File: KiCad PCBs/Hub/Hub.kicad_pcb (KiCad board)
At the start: 2 copper layers, 113.7 x 55.2 mm, 31 parts, among them J1 Conn_02x04_Top_Bottom, J2 Conn_02x04_Top_Bottom, U1 L7805CV

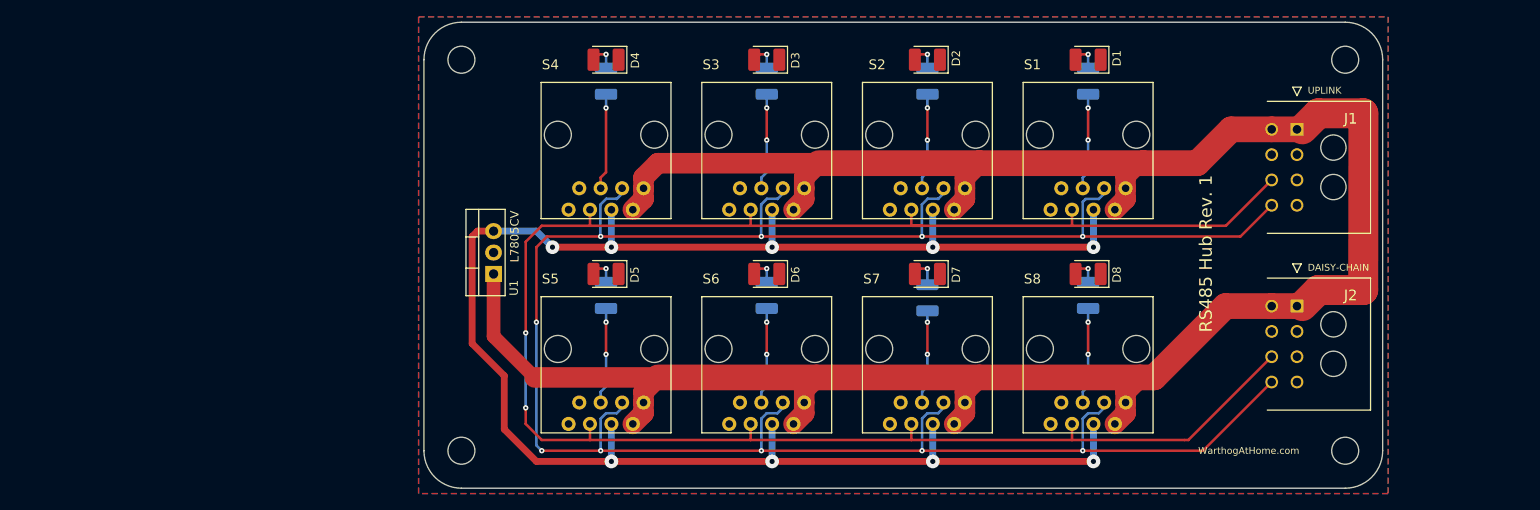
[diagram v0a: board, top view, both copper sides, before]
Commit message: First version of Hub completed
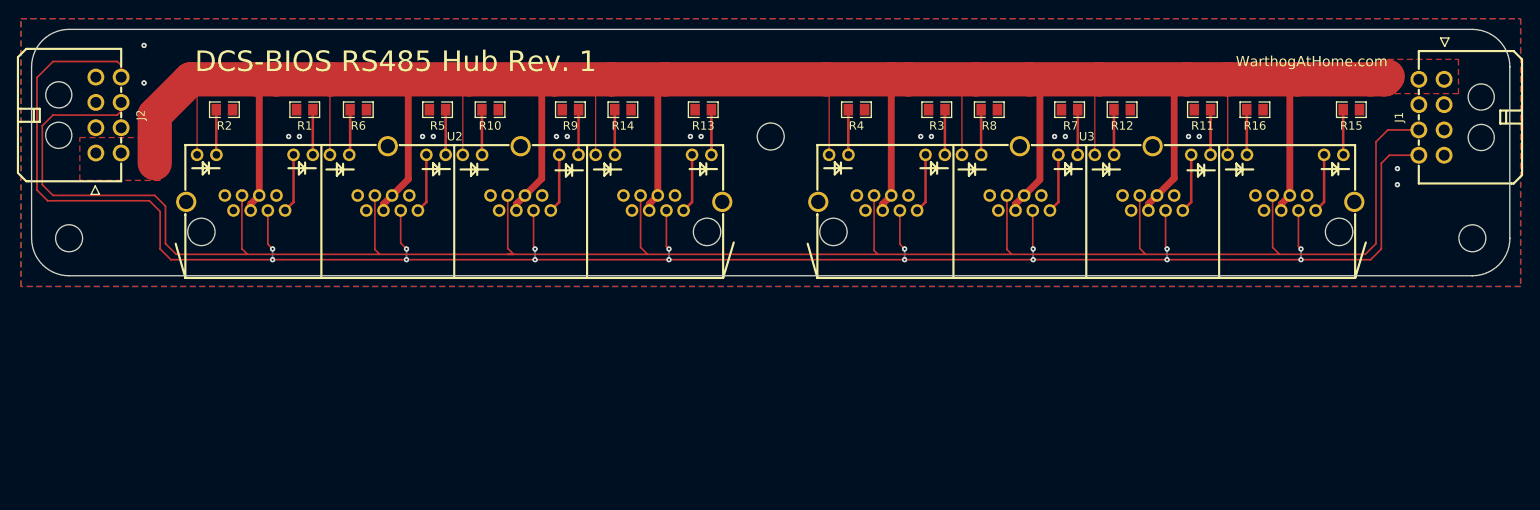
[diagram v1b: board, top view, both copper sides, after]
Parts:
- removed D1, D2, D3, D4, D5, D6, D7, D8: LED, LED_SMD:LED_1210_3225Metric_Pad1.42x2.65mm_HandSolder
- removed HOLE-1: MountingHole_3.2mm_M3, MountingHole:MountingHole_3.2mm_M3
- removed S1, S2, S3, S4, S5, S6, S7, S8: 8P8C, A10 KiCad Libraries:RJ45-8P8C
- removed U1: L7805CV, Package_TO_SOT_THT:TO-220-3_Vertical
- added R10: 1.8K, A10 KiCad Libraries:R0805, F.Cu at (112.6, 91.7)
- added R11: 390R, A10 KiCad Libraries:R0805, F.Cu at (197.1, 91.7)
- added R12: 1.8K, A10 KiCad Libraries:R0805, F.Cu at (187.5, 91.7)
- added R13: 390R, A10 KiCad Libraries:R0805, F.Cu at (137.9, 91.7)
- added R14: 1.8K, A10 KiCad Libraries:R0805, F.Cu at (128.4, 91.7)
- added R15: 390R, A10 KiCad Libraries:R0805, F.Cu at (214.7, 91.7)
- added R16: 1.8K, A10 KiCad Libraries:R0805, F.Cu at (203.3, 91.7)
- added R9: 390R, A10 KiCad Libraries:R0805, F.Cu at (122.1, 91.7)
- added U2: RJ45-B-1*4, A10 KiCad Libraries:RJ45-TH_B-1-4, F.Cu at (108.4, 103.7)
- added U3: RJ45-B-1*4, A10 KiCad Libraries:RJ45-TH_B-1-4, F.Cu at (183.4, 103.7)
- J1, J2: footprint A10 KiCad Libraries:Molex 43045-0800 -> A10 KiCad Libraries:Molex Micro-Fit 3.0 43045-0800
- R1, R3, R5, R7: value 400R -> 390R; footprint Resistor_SMD:R_1210_3225Metric_Pad1.30x2.65mm_HandSolder -> A10 KiCad Libraries:R0805; moved to F.Cu
- R2, R4, R6, R8: value 400R -> 1.8K; footprint Resistor_SMD:R_1210_3225Metric_Pad1.30x2.65mm_HandSolder -> A10 KiCad Libraries:R0805; moved to F.Cu
- moved J2 144.2 mm to (65.9, 92.3), turned to -90 degrees
- moved R1 92.9 mm to (90.6, 91.7), turned to 0 degrees
- moved R2 83.4 mm to (81.1, 91.7), turned to 180 degrees
- moved HOLE-2 68.7 mm to (145.9, 94.8)
- moved R6 53.2 mm to (97.0, 91.7), turned to 180 degrees
- moved HOLE-3 52.9 mm to (62.7, 106.9)
- moved R4 29.9 mm to (156.1, 91.7), turned to 180 degrees
- moved R5 29.7 mm to (106.4, 91.7), turned to 0 degrees
- moved HOLE-4 29.4 mm to (229.1, 106.9)
- moved R7 27.9 mm to (181.3, 91.7), turned to 0 degrees
- moved R8 24.9 mm to (171.8, 91.7), turned to 180 degrees
- moved R3 20.4 mm to (165.6, 91.7), turned to 0 degrees
- moved J1 17.5 mm to (225.7, 92.5)
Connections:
- net RS485-A renamed RS485+
- net RS485-B renamed RS485-
- R1 pad 1: 5V_S1 -> GND
- R2 pad 1: 5V_S2 -> GND
- R3 pad 1: 5V_S3 -> GND
- R4 pad 1: 5V_S4 -> GND
- R5 pad 1: 5V_S5 -> GND
- R6 pad 1: 5V_S6 -> GND
- R7 pad 1: 5V_S7 -> GND
- R8 pad 1: 5V_S8 -> GND
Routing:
- net 5V: track 206.1 -> 0.00 mm, vias 9 -> 0
- net 12V: track 278.2 -> 365.6 mm
- net RS485-: track 222.9 -> 259.2 mm, vias 2 -> 0
- net RS485+: track 263.9 -> 254.5 mm, vias 10 -> 16
- net Net-(R15-Pad2): track 0.00 -> 5.36 mm
- net Net-(R16-Pad2): track 0.00 -> 5.36 mm
- net Net-(R14-Pad2): track 0.00 -> 5.36 mm
- net Net-(R12-Pad2): track 0.00 -> 5.36 mm
- net Net-(R10-Pad2): track 0.00 -> 5.36 mm
- net Net-(R9-Pad2): track 0.00 -> 5.35 mm
- net Net-(R11-Pad2): track 0.00 -> 5.35 mm
- net Net-(R13-Pad2): track 0.00 -> 5.35 mm
- net 5V_S4: track 11.4 -> 7.01 mm, vias 1 -> 0
- net 5V_S2: track 11.4 -> 7.01 mm, vias 2 -> 0
- net 5V_S1: track 11.4 -> 7.01 mm, vias 2 -> 0
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- added copper zone on F.Cu, net 12V
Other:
- board size 113.7 x 55.2 mm -> 175.3 x 29.2 mm
- rule pad_to_mask_clearance: 0.0508 -> 0
- board text added: "DCS-BIOS RS485 Hub Rev. 1"
- board text removed: "RS485 Hub Rev. 1"
